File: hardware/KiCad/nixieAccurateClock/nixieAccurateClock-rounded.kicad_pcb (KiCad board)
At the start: 4 copper layers, 152.4 x 101.6 mm, 102 parts, among them J1 Conn_01x02_Pin, J10 Conn_01x02_Pin, J17 Conn_02x05_Odd_Even, J2 Conn_01x02_Pin, J3 Conn_01x02_Pin, J4 pico iCE (A), J5 pico iCE (B), J6 Conn_01x02_Pin, J7 Conn_01x02_Pin, J8 Conn_Coaxial, J9 Conn_01x02_Pin, Q1 PZTA42, Q2 PZTA42, Q3 PZTA42, Q4 PZTA42, Q5 PZTA42, Q6 PZTA42, SW1 SW_DIP_x08, U1 MCP23008-xSO, U2 LTR-329ALS-01, U3 PX1125T, U6 ADC0820BCWMX

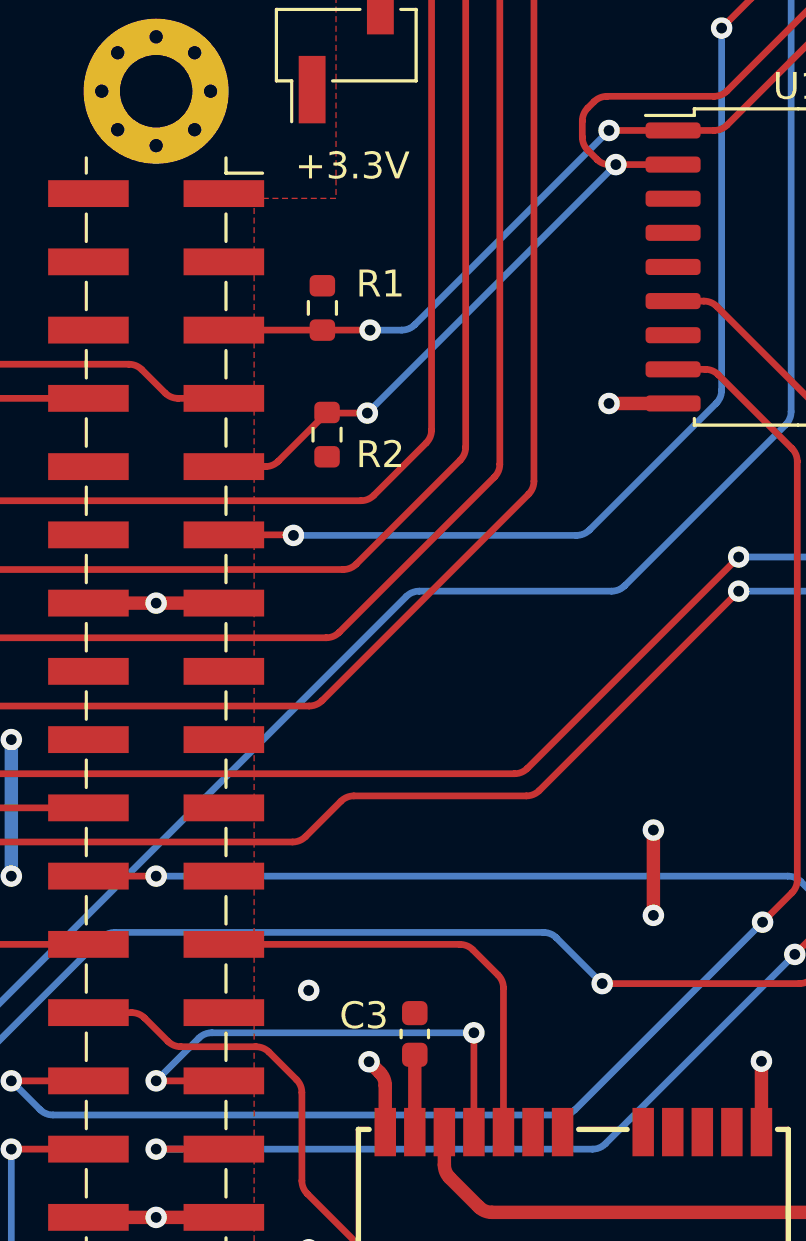
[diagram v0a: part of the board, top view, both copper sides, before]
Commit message: Update date
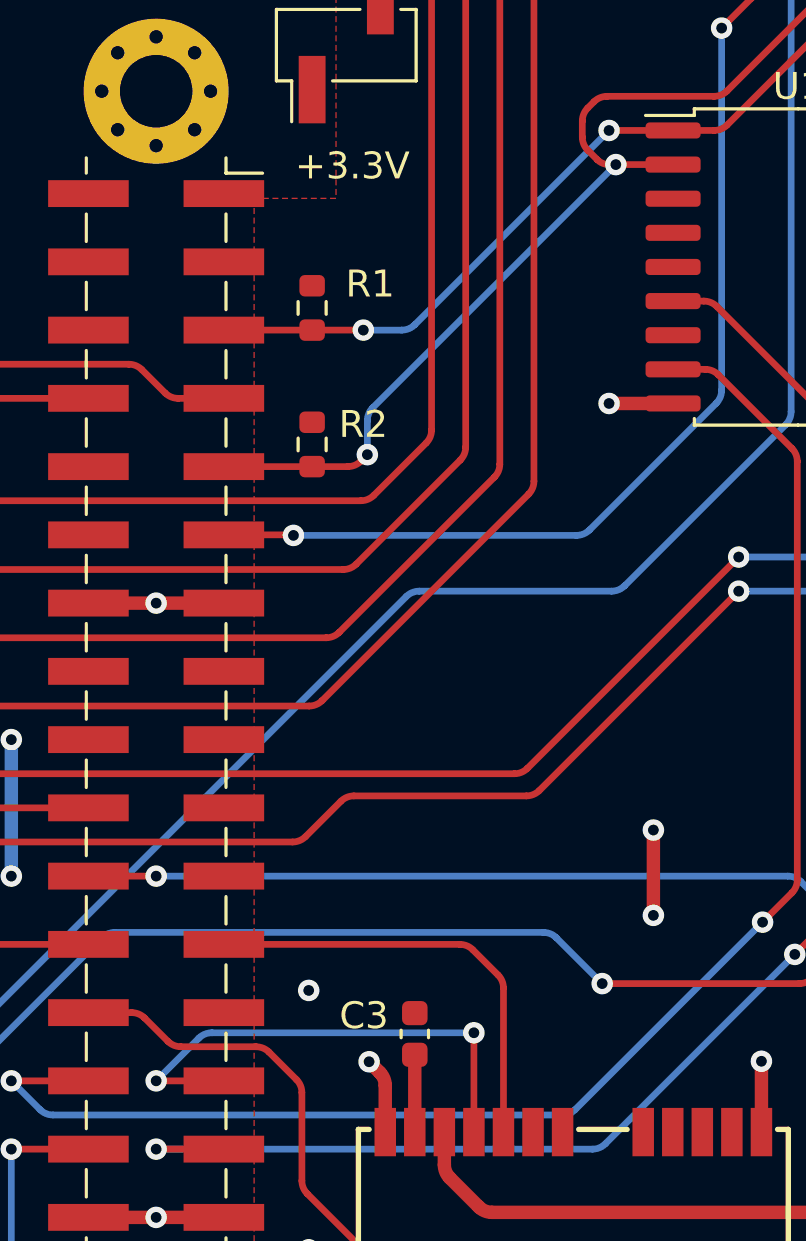
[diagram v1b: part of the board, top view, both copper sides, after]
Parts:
- moved R2 0.66 mm to (115.6, 70.7), turned to 90 degrees
- moved R1 0.38 mm to (115.6, 65.7)
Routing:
- net I2C_{CLOCK}: track 70.3 -> 69.0 mm
- net I2C_{DATA}: track 74.8 -> 75.7 mm
